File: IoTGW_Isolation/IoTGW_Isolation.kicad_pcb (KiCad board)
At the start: 4 copper layers, 60 x 45 mm, 31 parts, among them J4 39502-1008, J5 39502-1008, U1 TEA1-0505, U2 ISO1452BDWR, U3 LTV-817S, U4 LTV-817S, U5 LTV-817S, U6 LTV-817S, U7 LTV-817S, U8 LTV-817S

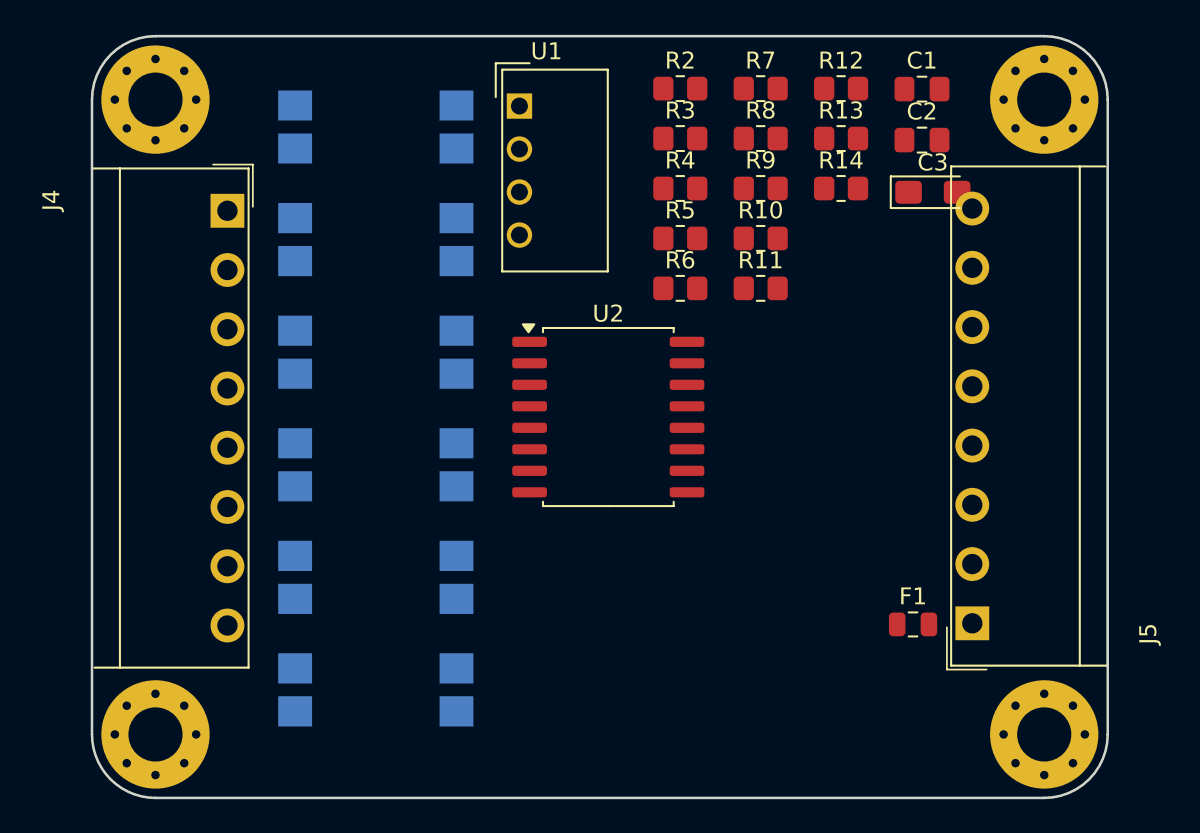
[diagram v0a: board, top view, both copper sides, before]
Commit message: PCB update
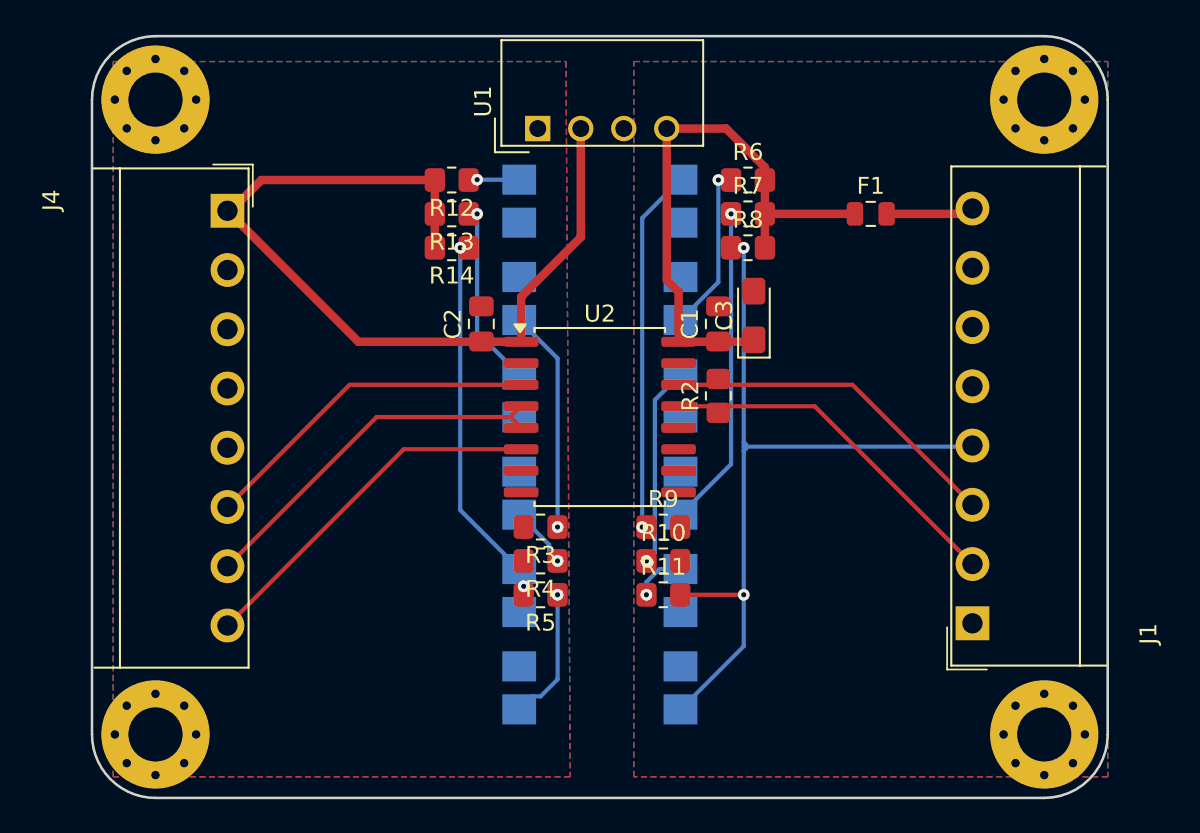
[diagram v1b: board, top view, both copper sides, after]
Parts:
- removed J5: 39502-1008, IoTGW:Molex_8pin_3.50
- added J1: 39502-1008, IoTGW:Molex_8pin_3.50, F.Cu at (174.9, 127.2)
- moved C2 28.2 mm to (138.0, 107.0), turned to 90 degrees
- moved R3 24.4 mm to (141.5, 119.0), turned to 180 degrees
- moved F1 24.4 mm to (161.0, 100.5)
- moved U5 23.8 mm to (145.0, 128.5), turned to 0 degrees
- moved R12 23.6 mm to (136.2, 98.5), turned to 180 degrees
- moved R4 23.5 mm to (141.5, 121.0), turned to 180 degrees
- moved R13 23.4 mm to (136.2, 100.5), turned to 180 degrees
- moved R14 23.3 mm to (136.2, 102.5), turned to 180 degrees
- moved R5 22.6 mm to (141.5, 123.0), turned to 180 degrees
- moved R9 20.8 mm to (148.8, 119.0)
- moved U6 20.4 mm to (145.0, 99.8)
- moved U4 20.0 mm to (145.0, 117.0), turned to 0 degrees
- moved R10 19.9 mm to (148.8, 121.0)
- moved R11 19.0 mm to (148.8, 123.0)
- moved C1 18.4 mm to (152.0, 107.0), turned to 90 degrees
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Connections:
- C1 pad 1: +5V_PROT -> +5V_OUT
- C3 pad 1: +5V_PROT -> +5V_OUT
- J4 pad 6: GPIO_COMM -> GPIO_R
- J4 pad 7: GPIO_R -> GPIO_COMM
- R12 pad 2: +5V_PROT -> +5V
- R13 pad 2: +5V_PROT -> +5V
- R14 pad 2: +5V_PROT -> +5V
- R6 pad 2: +5V_PROT -> +5V_OUT
- R7 pad 2: +5V_PROT -> +5V_OUT
- R8 pad 2: +5V_PROT -> +5V_OUT
- U2 pad 16: +5V_PROT -> +5V_OUT
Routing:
- net +5V: track 0.00 -> 51.6 mm
- net GPIO_EXT_2: track 0.00 -> 46.6 mm, vias 0 -> 2
- net +5V_OUT: track 0.00 -> 34.2 mm
- net GPIO_COMM: track 0.00 -> 22.2 mm
- net GPIO_D: track 0.00 -> 21.7 mm
- net GPIO_OPTO_2: track 0.00 -> 21.6 mm, vias 0 -> 2
- net Net-(R9-Pad1): track 0.00 -> 21.5 mm, vias 0 -> 1
- net RS-485_B: track 0.00 -> 21.2 mm
- net GPIO_R: track 0.00 -> 20.3 mm
- net RS-485_A: track 0.00 -> 20.3 mm
- net GPIO_EXT_1: track 0.00 -> 19.0 mm, vias 0 -> 1
- net Net-(R3-Pad1): track 0.00 -> 13.2 mm, vias 0 -> 1
- net Net-(R10-Pad1): track 0.00 -> 11.9 mm, vias 0 -> 1
- net GPIO_OPTO_1: track 0.00 -> 10.5 mm, vias 0 -> 1
- net GPIO_EXT_0: track 0.00 -> 9.20 mm, vias 0 -> 1
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- added copper zone on B.Cu, net GND
- added copper zone on F.Cu, net GND
- added copper zone on B.Cu, net GND_OUT
- added copper zone on F.Cu, net GND_OUT
